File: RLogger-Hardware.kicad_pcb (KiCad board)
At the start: 2 copper layers, 13 parts, among them J1 Bat Connector, J2 Baro, J3 FRAM, J4 MicroSD, J5 BMI160, U1 MIC2288BD5

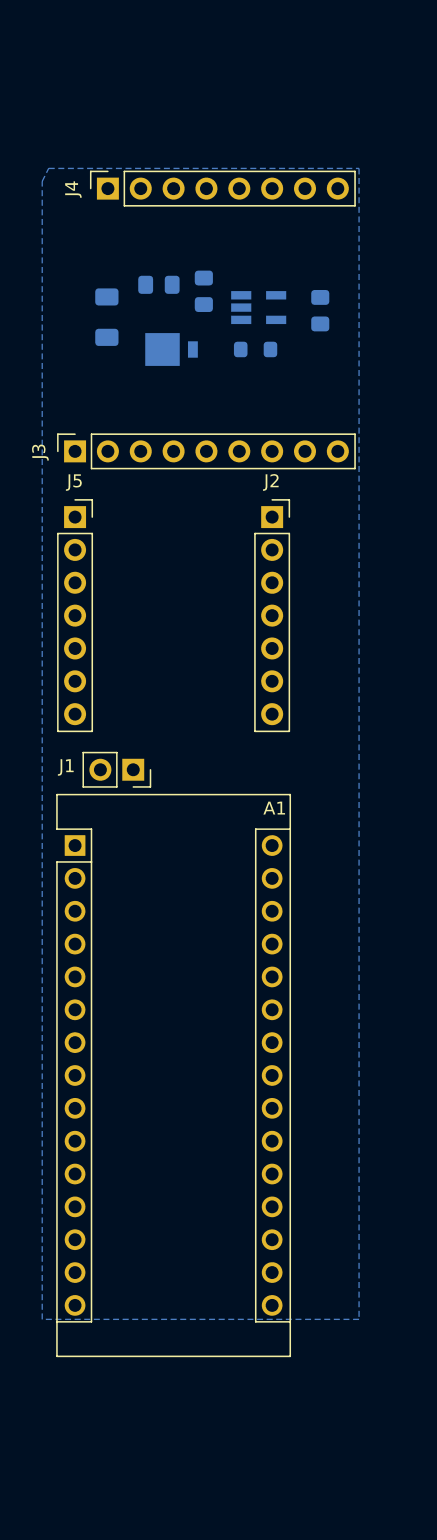
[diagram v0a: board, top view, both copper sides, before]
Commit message: PCB done :o
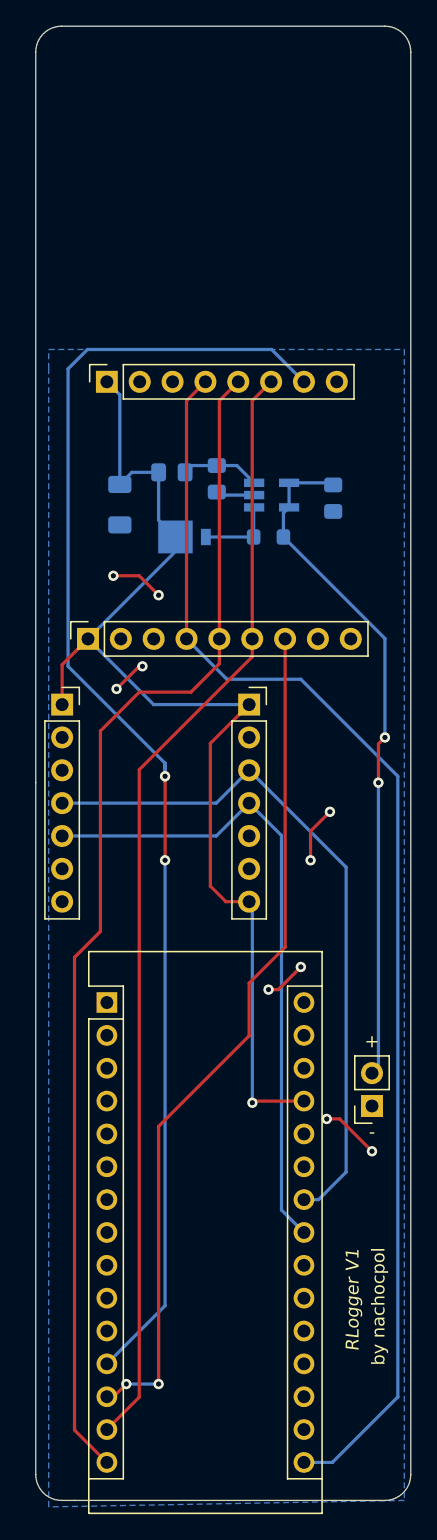
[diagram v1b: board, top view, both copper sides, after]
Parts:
- moved J1 31.9 mm to (152.5, 106.5), turned to 180 degrees
- moved J4 14.9 mm to (132.0, 50.5)
- moved J2 14.6 mm to (143.0, 75.5)
- moved C1 14.5 mm to (149.5, 59.5)
- moved C2 14.5 mm to (133.0, 60.0)
- moved D1 14.5 mm to (138.0, 62.5)
- moved L1 14.5 mm to (144.5, 62.5)
- moved R1 14.5 mm to (137.0, 57.5)
- moved R2 14.5 mm to (140.5, 58.0)
- moved U1 14.5 mm to (144.7, 59.3)
- moved J3 14.5 mm to (130.5, 70.4)
- moved J5 14.5 mm to (128.5, 75.5)
- moved A1 12.4 mm to (132.0, 98.5)
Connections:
- A1 pad 12: /CS -> /SS1
- A1 pad 13: /CS -> /SS0
- A1 pad 27: /+5V5 -> /+5V
- C2 pad 1: /+5V5 -> /+5V
- D1 pad 1: /+5V5 -> /+5V
- J2 pad 1: /+5V5 -> /+5V
- J2 pad 7: /+5V5 -> /+5V
- J3 pad 7: /CS -> /SS0
- J4 pad 7: /CS -> /SS1
- R1 pad 1: /+5V5 -> /+5V
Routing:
- net /SS1: track 0.00 -> 103.3 mm, vias 0 -> 2
- net /SCK: track 0.00 -> 98.6 mm
- net /DO: track 0.00 -> 92.2 mm
- net /+5V: track 0.00 -> 86.9 mm, vias 0 -> 1
- net /DI: track 0.00 -> 86.3 mm
- net /SS0: track 0.00 -> 66.1 mm, vias 0 -> 2
- net /SCL: track 0.00 -> 53.8 mm
- net +BATT: track 0.00 -> 53.0 mm, vias 0 -> 2
- net /SDA: track 0.00 -> 50.5 mm
- net GND: track 0.00 -> 22.0 mm, vias 0 -> 10
- net Net-(R1-Pad2): track 0.00 -> 6.11 mm
- net Net-(D1-Pad2): track 0.00 -> 6.00 mm
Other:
- board outline added: 29 x 114 mm
- board text added: "+"
- board text added: "-"
- board text added: "RLogger V1"
- board text added: "by nachocpol"
